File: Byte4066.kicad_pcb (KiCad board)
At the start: 2 copper layers, 4 parts, among them J1 Conn_01x10, J2 Conn_02x08_Odd_Even, U1 4066, U2 4066

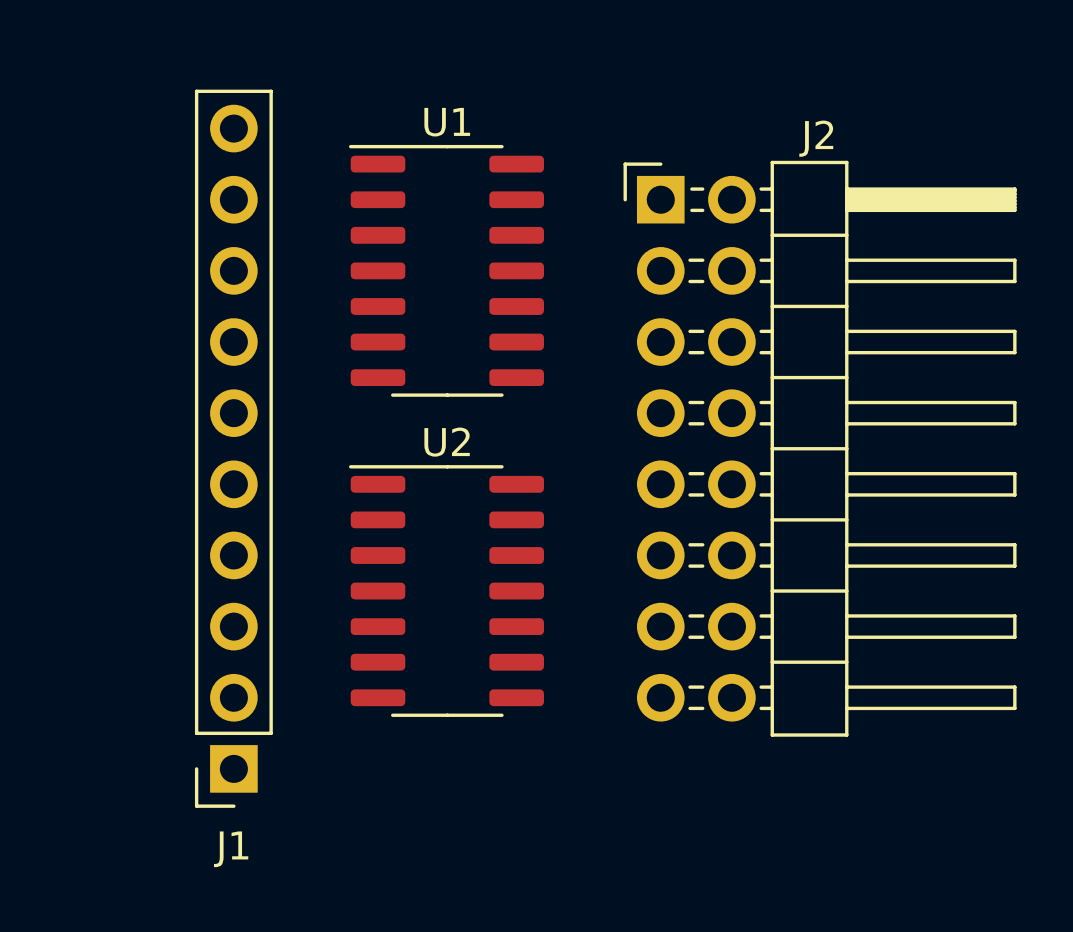
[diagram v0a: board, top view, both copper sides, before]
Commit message: V1
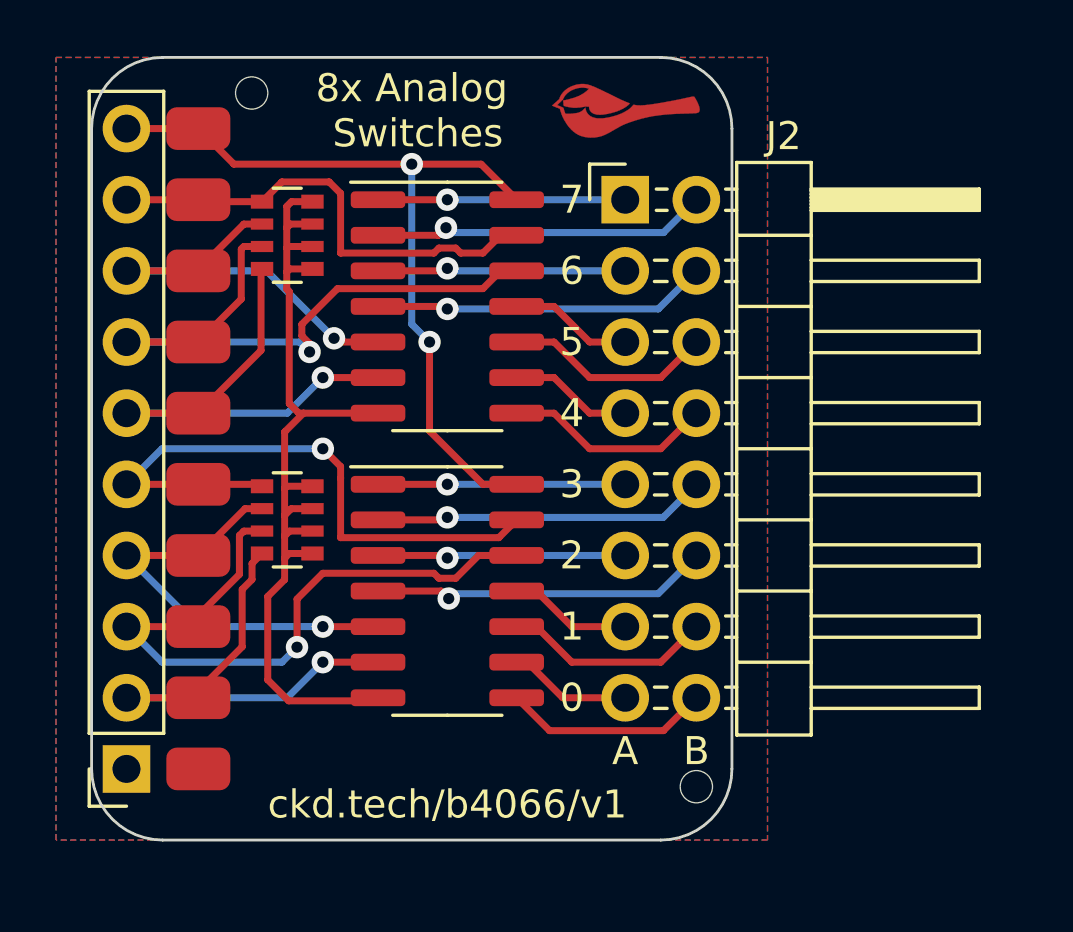
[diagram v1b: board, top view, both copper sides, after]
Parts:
- added G***: LOGO, chickadee:chickadee_2mm_fcu, F.Cu at (152.4, 88.3)
- added J3: Conn_01x10, pads:1x10 pads, F.Cu at (137.2, 100.3)
- added REF**: ToolingHole, JLCPCB:ToolingHole, F.Cu at (154.9, 112.4)
- added REF**: ToolingHole, JLCPCB:ToolingHole, F.Cu at (139.1, 87.6)
- added RN1: R_Pack04, Resistor_SMD:R_Array_Convex_4x0603, F.Cu at (140.3, 102.9)
- added RN2: R_Pack04, Resistor_SMD:R_Array_Convex_4x0603, F.Cu at (140.3, 92.7)
- moved J1 3.84 mm to (134.6, 111.8)
- moved U1 1.27 mm to (146.1, 95.2)
- moved J2 1.27 mm to (152.4, 91.4)
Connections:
- J2 pad 1: unconnected-(J2-Pad1) -> /7A
- J2 pad 10: unconnected-(J2-Pad10) -> /3B
- J2 pad 11: unconnected-(J2-Pad11) -> /2A
- J2 pad 12: unconnected-(J2-Pad12) -> /2B
- J2 pad 2: unconnected-(J2-Pad2) -> /7B
- J2 pad 3: unconnected-(J2-Pad3) -> /6A
- J2 pad 4: unconnected-(J2-Pad4) -> /6B
- J2 pad 5: unconnected-(J2-Pad5) -> /5A
- J2 pad 6: unconnected-(J2-Pad6) -> /5B
- J2 pad 7: unconnected-(J2-Pad7) -> /4A
- J2 pad 8: unconnected-(J2-Pad8) -> /4B
- J2 pad 9: unconnected-(J2-Pad9) -> /3A
- U1 pad 1: unconnected-(U1-Pad1) -> /7A
- U1 pad 10: unconnected-(U1-Pad10) -> /5B
- U1 pad 11: unconnected-(U1-Pad11) -> /5A
- U1 pad 12: unconnected-(U1-Pad12) -> /P5
- U1 pad 13: unconnected-(U1-Pad13) -> /P7
- U1 pad 2: unconnected-(U1-Pad2) -> /7B
- U1 pad 3: unconnected-(U1-Pad3) -> /6A
- U1 pad 4: unconnected-(U1-Pad4) -> /6B
- U1 pad 5: unconnected-(U1-Pad5) -> /P6
- U1 pad 6: unconnected-(U1-Pad6) -> /P4
- U1 pad 8: unconnected-(U1-Pad8) -> /4B
- U1 pad 9: unconnected-(U1-Pad9) -> /4A
- U2 pad 1: unconnected-(U2-Pad1) -> /3A
- U2 pad 13: unconnected-(U2-Pad13) -> /P3
- U2 pad 2: unconnected-(U2-Pad2) -> /3B
- U2 pad 3: unconnected-(U2-Pad3) -> /2A
- U2 pad 4: unconnected-(U2-Pad4) -> /2B
- U2 pad 5: unconnected-(U2-Pad5) -> /P2
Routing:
- net GND: track 0.00 -> 32.8 mm
- net VCC: track 0.00 -> 28.7 mm, vias 0 -> 2
- net /P1: track 0.00 -> 24.5 mm, vias 0 -> 1
- net /P5: track 0.00 -> 23.5 mm, vias 0 -> 1
- net /P3: track 0.00 -> 22.4 mm, vias 0 -> 1
- net /P4: track 0.00 -> 18.2 mm, vias 0 -> 1
- net /P0: track 0.00 -> 18.2 mm, vias 0 -> 1
- net /P7: track 0.00 -> 17.0 mm
- net /P6: track 0.00 -> 15.6 mm, vias 0 -> 1
- net /P2: track 0.00 -> 15.6 mm, vias 0 -> 1
- net /2B: track 0.00 -> 12.4 mm, vias 0 -> 1
- net /7B: track 0.00 -> 12.3 mm, vias 0 -> 1
- net /6B: track 0.00 -> 12.0 mm, vias 0 -> 1
- net /3B: track 0.00 -> 11.9 mm, vias 0 -> 1
- net /6A: track 0.00 -> 8.90 mm, vias 0 -> 1
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- added copper zone on B.Cu, net GND
- added copper zone on F.Cu, net GND
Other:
- board outline added: 22.9 x 27.9 mm
- board text added: "0"
- board text added: "1"
- board text added: "2"
- board text added: "3"
- board text added: "4"
- board text added: "5"
- board text added: "6"
- board text added: "7"
- board text added: "8x Analog Switches"
- board text added: "A"
- board text added: "B"
- board text added: "JLCJLCJLCJLC"
- board text added: "ckd.tech/b4066/v1"
